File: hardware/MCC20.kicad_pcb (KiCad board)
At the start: 2 copper layers, 247.1 x 121 mm, 212 parts, among them J1 Conn_01x04, J401 USART, J601 RJ45, J602 RJ45, U201 MCP2551-I/SN, U202 MCP2515-xSO, U401 ATMEGA328P-PU, U501 LM7805, Y201 16MHz, Y401 16MHz

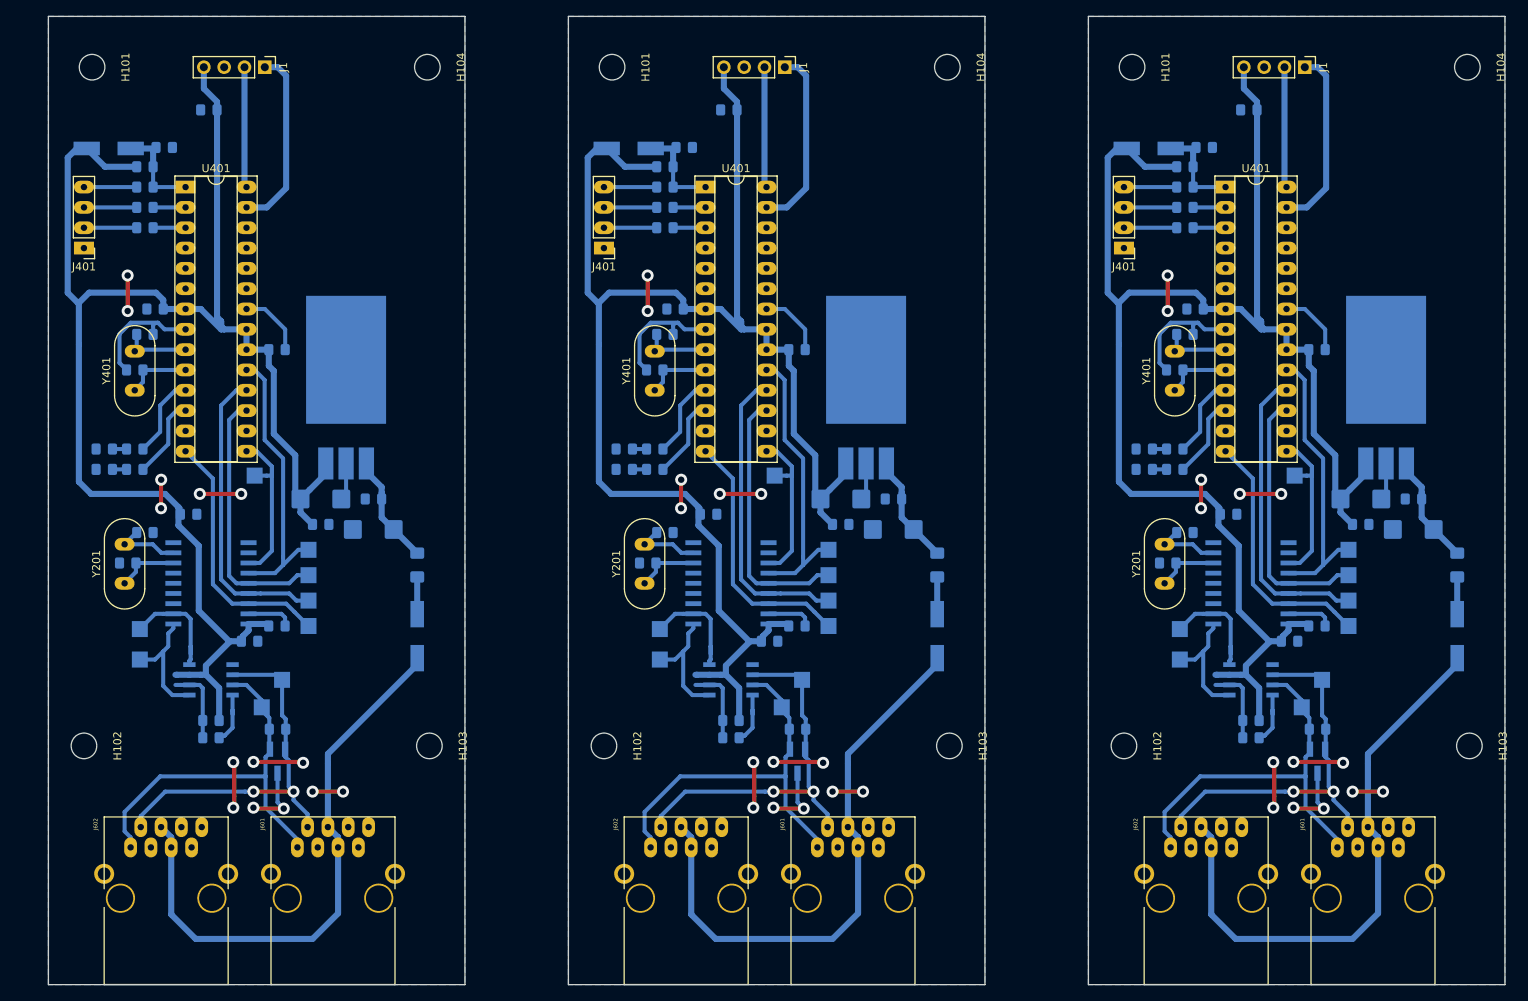
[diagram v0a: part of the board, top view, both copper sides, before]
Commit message: Signal and Cuk imported
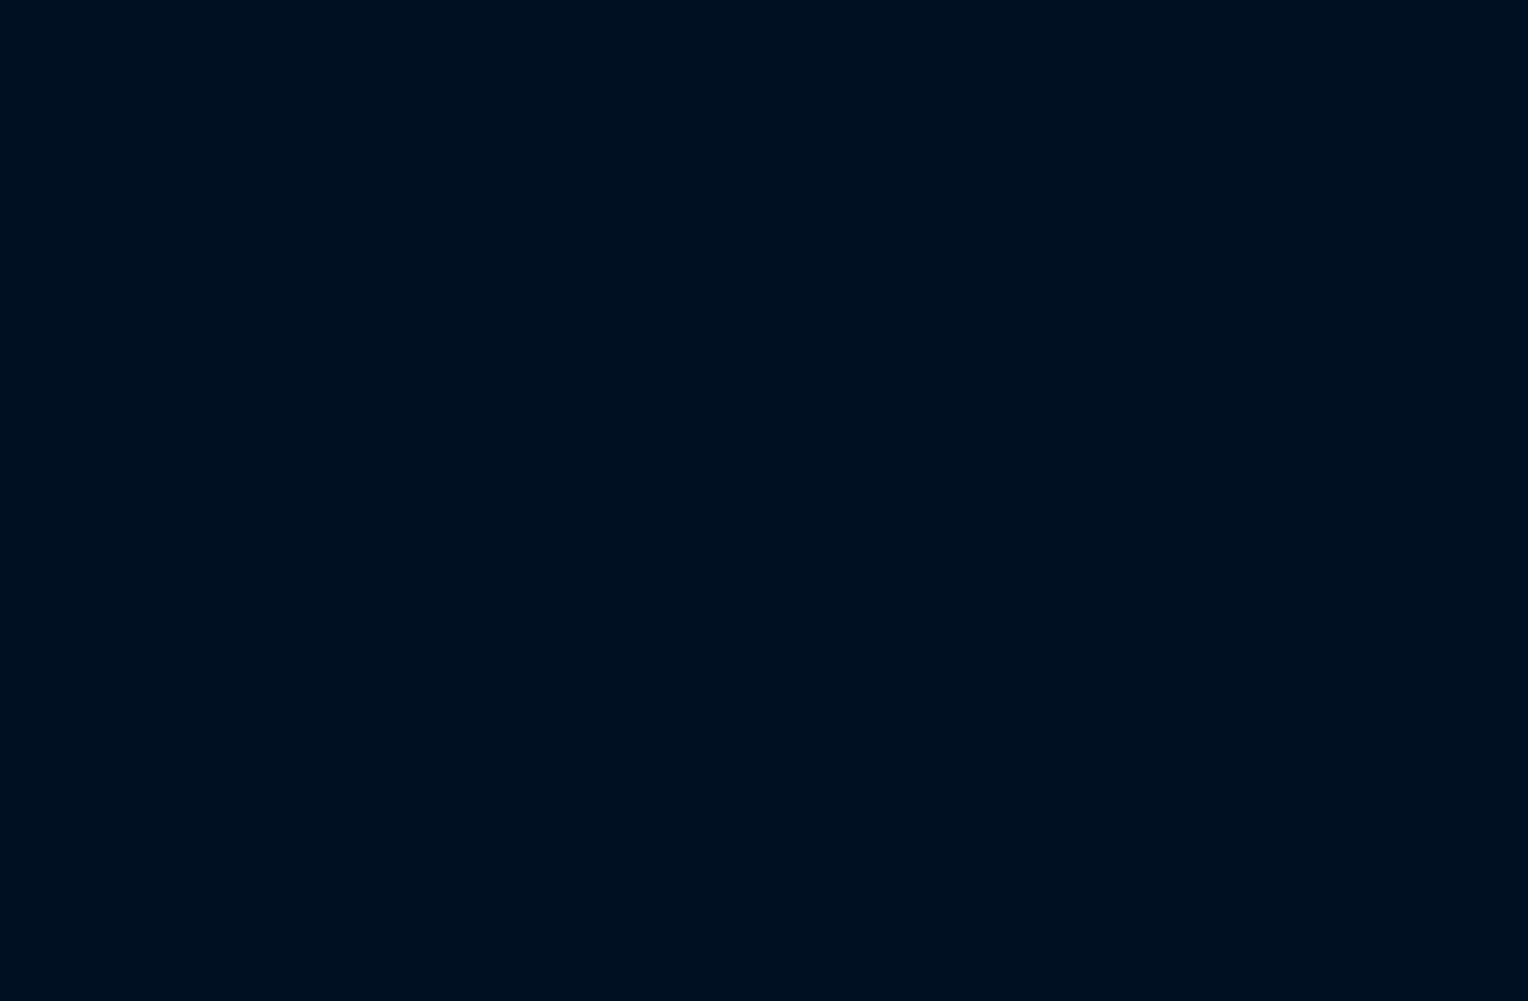
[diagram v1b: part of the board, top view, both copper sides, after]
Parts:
- removed the C102 at (237.5, 43.4)
- removed the C102 at (172.5, 43.4)
- removed the C102 at (107.5, 43.4)
- removed the C201 at (235.0, 94.0)
- removed the C201 at (170.0, 94.0)
- removed the C201 at (105.0, 94.0)
- removed the C202 at (242.6, 109.9)
- removed the C202 at (177.6, 109.9)
- removed the C202 at (112.6, 109.9)
- removed the C203 at (227.4, 100.1)
- removed the C203 at (162.4, 100.1)
- removed the C203 at (97.4, 100.1)
- removed the C204 at (229.5, 96.3)
- removed the C204 at (164.5, 96.3)
- removed the C204 at (99.5, 96.3)
- removed the C205 at (237.8, 119.8)
- removed the C205 at (172.8, 119.8)
- removed the C205 at (107.8, 119.8)
- removed the C401 at (246.1, 73.4)
- removed the C401 at (181.1, 73.4)
- removed the C401 at (116.1, 73.4)
- removed the C402 at (230.8, 68.3)
- removed the C402 at (165.8, 68.3)
- removed the C402 at (100.8, 68.3)
- removed the C403 at (228.3, 75.9)
- removed the C403 at (163.3, 75.9)
- removed the C403 at (98.3, 75.9)
- removed the C404 at (229.5, 71.5)
- removed the C404 at (164.5, 71.5)
- removed the C404 at (99.5, 71.5)
- removed the C405 at (229.5, 53.1)
- removed the C405 at (164.5, 53.1)
- removed the C405 at (99.5, 53.1)
- removed the C406 at (232.0, 48.1)
- removed the C406 at (167.0, 48.1)
- removed the C406 at (102.0, 48.1)
- removed the C501 at (258.1, 95.9)
- removed the C501 at (193.1, 95.9)
- removed the C501 at (128.1, 95.9)
- removed the C502 at (258.1, 92.1)
- removed the C502 at (193.1, 92.1)
- removed the C502 at (128.1, 92.1)
- removed the C503 at (251.5, 95.2)
- removed the C503 at (186.5, 95.2)
- removed the C503 at (121.5, 95.2)
- removed the C504 at (251.5, 92.1)
- removed the C504 at (186.5, 92.1)
- removed the C504 at (121.5, 92.1)
- removed the D201 at (246.1, 124.8)
- removed the D201 at (181.1, 124.8)
- removed the D201 at (116.1, 124.8)
- removed the D401 at (225.0, 48.3)
- removed the D401 at (160.0, 48.3)
- removed the D401 at (95.0, 48.3)
- removed the D402 at (224.5, 88.4)
- removed the D402 at (159.5, 88.4)
- removed the D402 at (94.5, 88.4)
- removed the D403 at (224.5, 85.8)
- removed the D403 at (159.5, 85.8)
- removed the D403 at (94.5, 85.8)
- removed the D501 at (263.6, 109.2)
- removed the D501 at (198.6, 109.2)
- removed the D501 at (133.6, 109.2)
- removed the F501 at (263.6, 100.3)
- removed the F501 at (198.6, 100.3)
- removed the F501 at (133.6, 100.3)
- removed the H101 at (222.9, 38.1)
- removed the H101 at (157.9, 38.1)
- removed the H101 at (92.9, 38.1)
- removed the H102 at (221.9, 122.9)
- removed the H102 at (156.9, 122.9)
- removed the H102 at (91.9, 122.9)
- removed the H103 at (265.1, 122.9)
- removed the H103 at (200.1, 122.9)
- removed the H103 at (135.1, 122.9)
- removed the H104 at (264.9, 38.1)
- removed the H104 at (199.8, 38.1)
- removed the H104 at (134.8, 38.1)
- removed the J1 at (244.5, 38.1)
- removed the J1 at (179.5, 38.1)
- removed the J1 at (114.5, 38.1)
- removed the J401 at (221.9, 60.7)
- removed the J401 at (156.9, 60.7)
- removed the J401 at (91.9, 60.7)
- removed the J601 at (248.6, 135.6)
- removed the J601 at (183.6, 135.6)
- removed the J601 at (118.6, 135.6)
- removed the J602 at (227.7, 135.6)
- removed the J602 at (162.7, 135.6)
- removed the J602 at (97.7, 135.6)
- removed the R201 at (246.1, 120.8)
- removed the R201 at (181.1, 120.8)
- removed the R201 at (116.1, 120.8)
- removed the R202 at (237.8, 121.9)
- removed the R202 at (172.8, 121.9)
- removed the R202 at (107.8, 121.9)
- removed the R203 at (246.0, 108.0)
- removed the R203 at (181.0, 108.0)
- removed the R203 at (116.0, 108.0)
- removed the R401 at (229.5, 50.5)
- removed the R401 at (164.5, 50.5)
- removed the R401 at (99.5, 50.5)
- removed the R402 at (229.5, 55.6)
- removed the R402 at (164.5, 55.6)
- removed the R402 at (99.5, 55.6)
- removed the R403 at (229.5, 58.2)
- removed the R403 at (164.5, 58.2)
- removed the R403 at (99.5, 58.2)
- removed the R404 at (228.3, 88.4)
- removed the R404 at (163.3, 88.4)
- removed the R404 at (98.3, 88.4)
- removed the R405 at (228.3, 85.8)
- removed the R405 at (163.3, 85.8)
- removed the R405 at (98.3, 85.8)
- removed the TP201 at (250.0, 101.6)
- removed the TP201 at (185.0, 101.6)
- removed the TP201 at (120.0, 101.6)
- removed the TP202 at (250.0, 104.8)
- removed the TP202 at (185.0, 104.8)
- removed the TP202 at (120.0, 104.8)
- removed the TP203 at (228.9, 112.1)
- removed the TP203 at (163.9, 112.1)
- removed the TP203 at (98.9, 112.1)
- removed the TP204 at (228.9, 108.3)
- removed the TP204 at (163.9, 108.3)
- removed the TP204 at (98.9, 108.3)
- removed the TP205 at (250.0, 108.0)
- removed the TP205 at (185.0, 108.0)
- removed the TP205 at (120.0, 108.0)
- removed the TP206 at (250.0, 98.4)
- removed the TP206 at (185.0, 98.4)
- removed the TP206 at (120.0, 98.4)
- removed the TP207 at (244.1, 118.1)
- removed the TP207 at (179.1, 118.1)
- removed the TP207 at (114.1, 118.1)
- removed the TP208 at (246.7, 114.7)
- removed the TP208 at (181.7, 114.7)
- removed the TP208 at (116.7, 114.7)
- removed the TP209 at (243.3, 89.2)
- removed the TP209 at (178.3, 89.2)
- removed the TP209 at (113.3, 89.2)
- removed the U201 at (237.8, 114.7)
- removed the U201 at (172.8, 114.7)
- removed the U201 at (107.8, 114.7)
- removed the U202 at (237.8, 102.6)
- removed the U202 at (172.8, 102.6)
- removed the U202 at (107.8, 102.6)
- removed the U401 at (234.6, 53.1)
- removed the U401 at (169.6, 53.1)
- removed the U401 at (104.6, 53.1)
- removed the U501 at (257.2, 86.4)
- removed the U501 at (192.2, 86.4)
- removed the U501 at (127.2, 86.4)
- removed the Y201 at (227.0, 102.6)
- removed the Y201 at (162.0, 102.6)
- removed the Y201 at (97.0, 102.6)
- removed the Y401 at (228.3, 78.5)
- removed the Y401 at (163.3, 78.5)
- removed the Y401 at (98.3, 78.5)
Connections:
- U501 pad : GND -> (no net)
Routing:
- net +5V: track 807.1 -> 201.8 mm
- net GND: track 318.1 -> 79.5 mm, vias 56 -> 14
- net /POWER SUPPLY/+18V_IN: track 287.8 -> 71.9 mm
- net /CANBUS CONN/CAN_H: track 202.3 -> 50.6 mm
- net /CANBUS CONN/CAN_L: track 192.7 -> 48.2 mm, vias 8 -> 2
- net /MISO: track 150.9 -> 37.7 mm
- net /SCK: track 142.3 -> 35.6 mm
- net /MOSI: track 131.5 -> 32.9 mm
- net /CANBUS/CS: track 128.6 -> 32.2 mm
- net /MCU/SDA: track 92.5 -> 23.1 mm
- net /CANBUS/INT: track 84.4 -> 21.1 mm
- net /CANBUS/TXCAN: track 61.4 -> 15.4 mm
- net /MCU/SCL: track 60.4 -> 15.1 mm
- net /CANBUS/RXCAN: track 56.5 -> 14.1 mm
- net /POWER SUPPLY/+18V_OUT: track 55.4 -> 13.8 mm
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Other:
- board size 247.1 x 121 mm -> 52.1 x 121 mm
